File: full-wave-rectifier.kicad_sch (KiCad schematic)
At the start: 40 parts, among them J10 Control Right, J11 Main Right, J2 Input Ch1, J3 Input Ch2, J4 Output Ch1, J5 Output Ch2, J6 Ochd input, J8 Control Left, J9 Main Left, U2 TL074, U3 TL074, U4 TL074

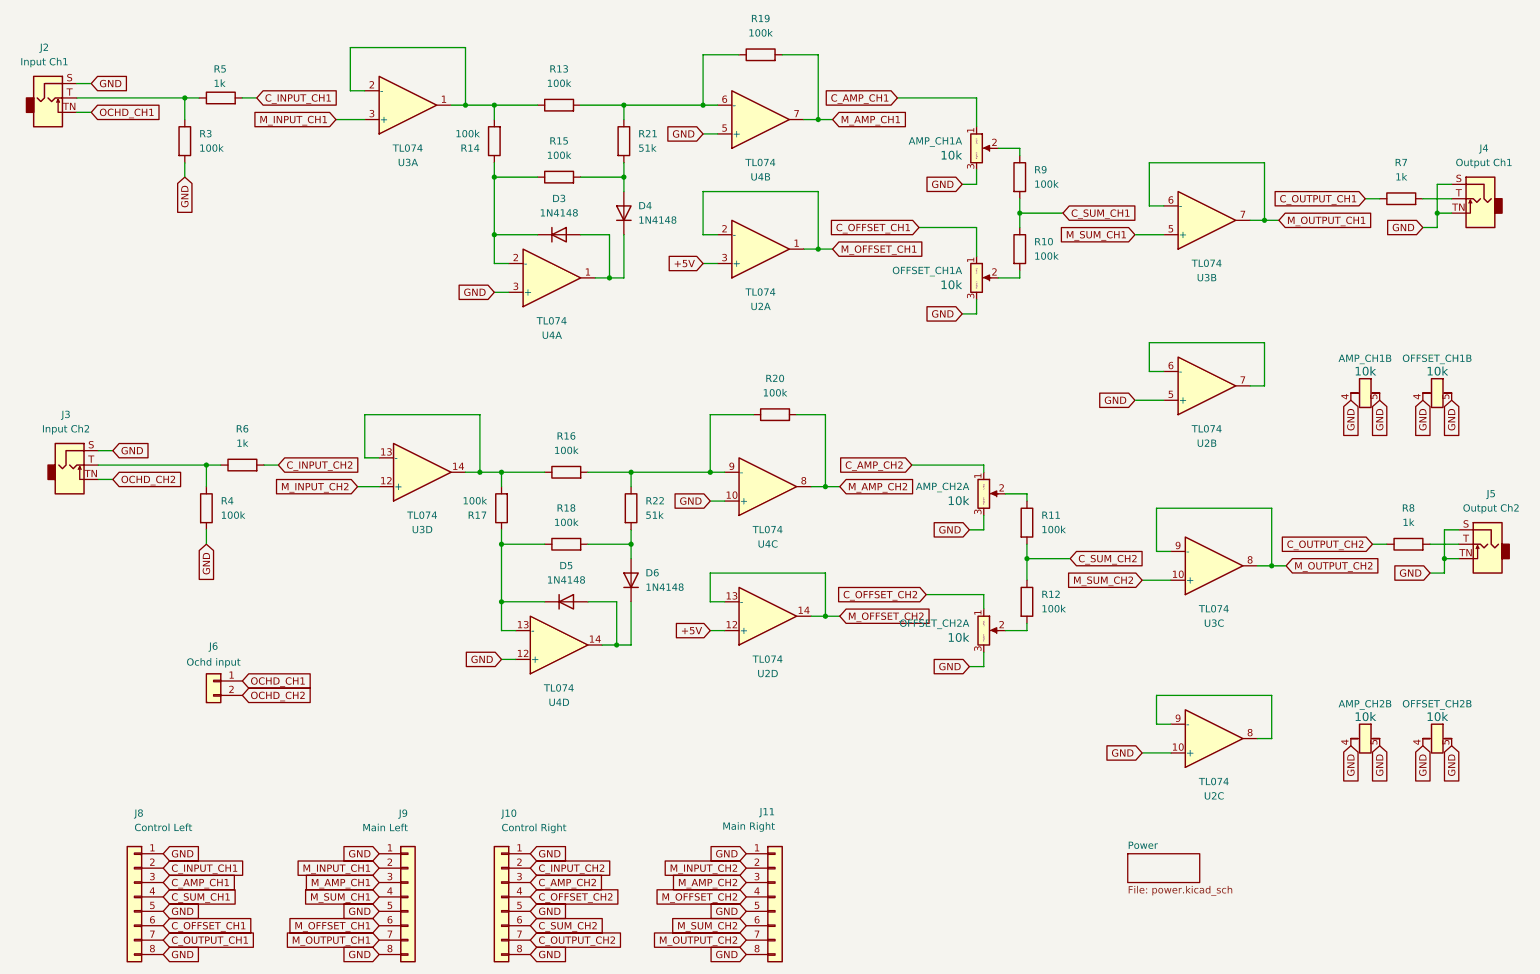
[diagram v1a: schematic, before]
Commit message: save chages
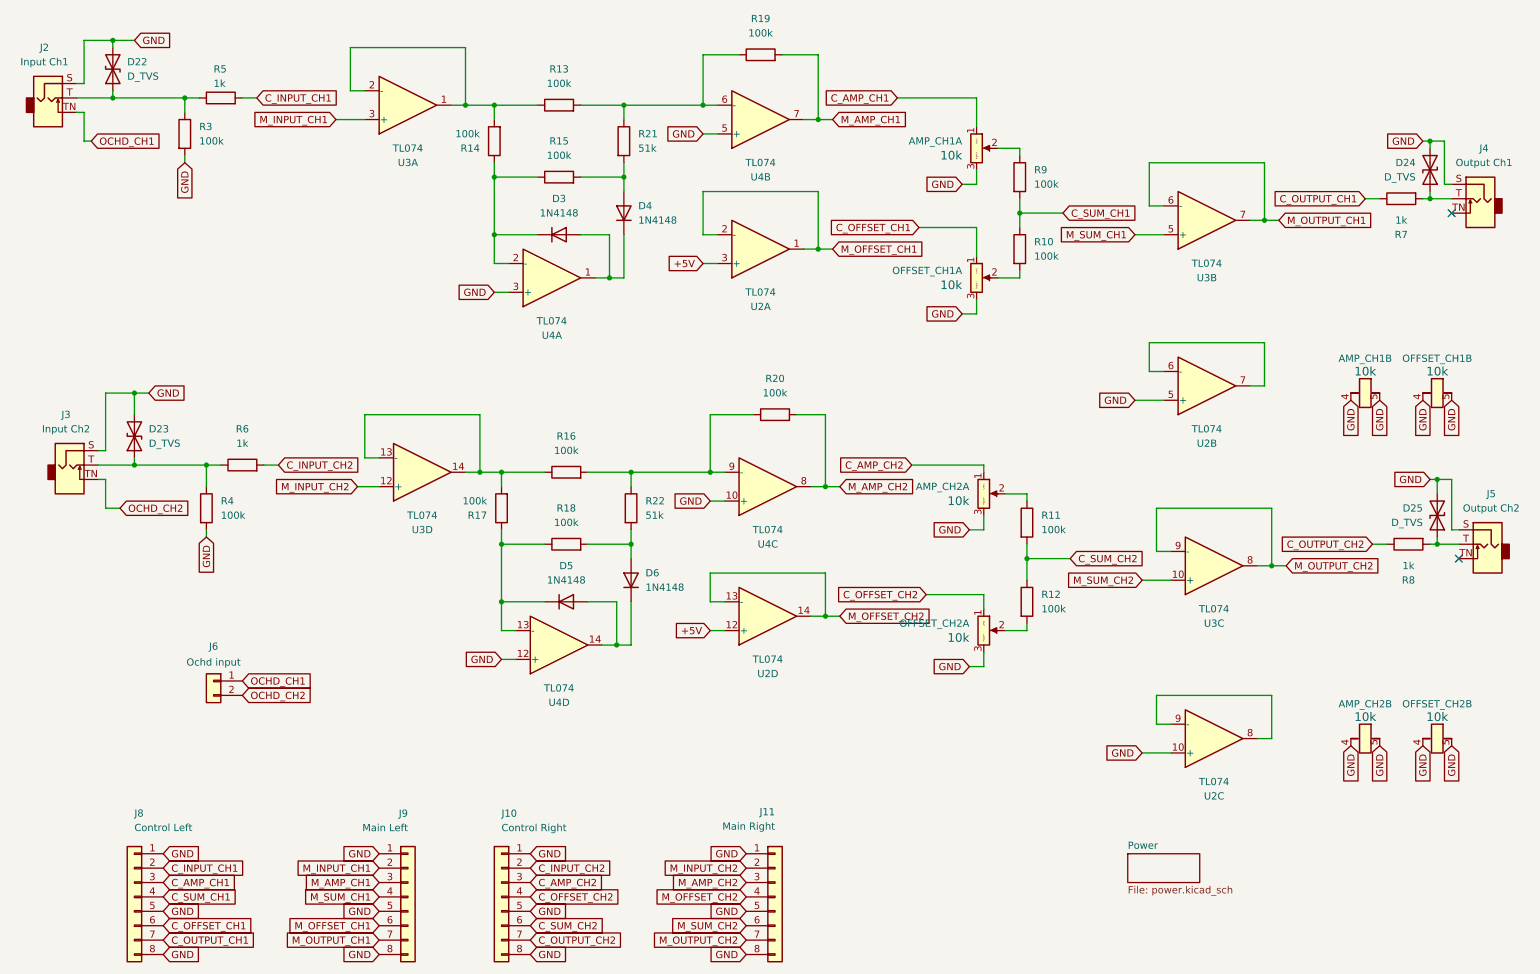
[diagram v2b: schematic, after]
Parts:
- added D22, D23, D24, D25: D_TVS, Diode_SMD:D_SOD-323_HandSoldering, symbol Device:D_TVS
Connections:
- net GND: now also D22.2 (A2), D23.2 (A2), D24.2 (A2), D25.2 (A2); no longer J4.TN, J5.TN
- net at J5.T, R8.2: now also D25.1 (A1)
- net at J3.T, R4.1, R6.1: now also D23.1 (A1)
- net at J2.T, R3.1, R5.1: now also D22.1 (A1)
- net at J4.T, R7.2: now also D24.1 (A1)
- no-connect marks 0 -> 2
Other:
- moved on the sheet: R3
